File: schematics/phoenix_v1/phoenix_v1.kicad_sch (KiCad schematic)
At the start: 1 part, among them U1 ESP32-DevKitC

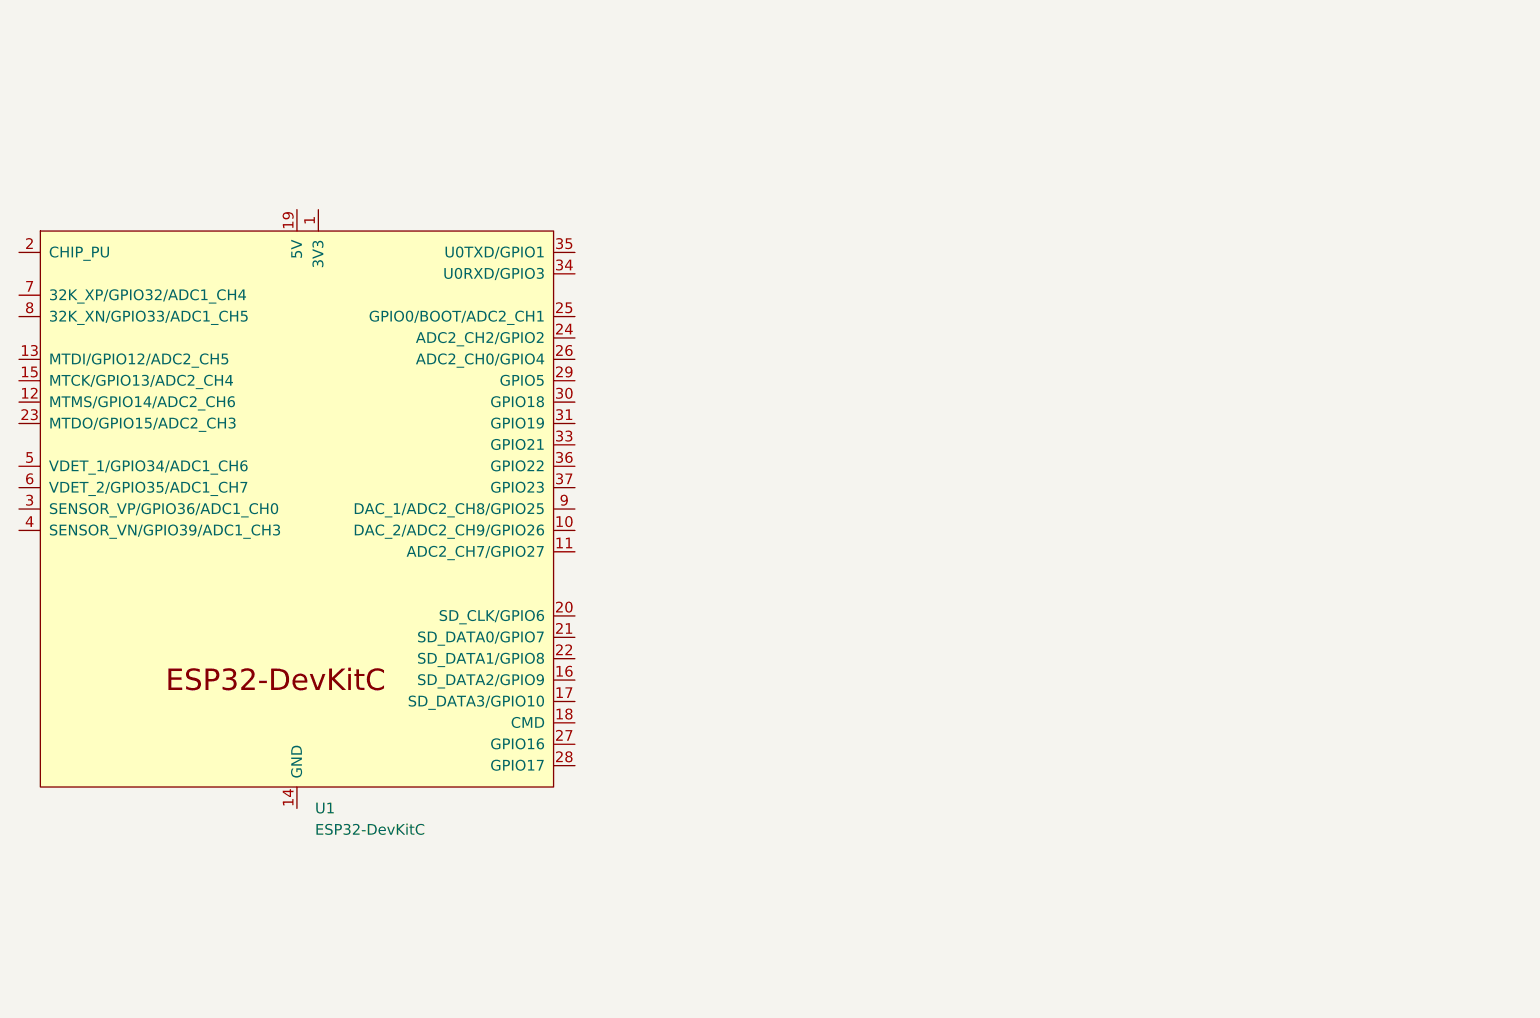
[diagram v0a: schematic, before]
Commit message: v1 schematic
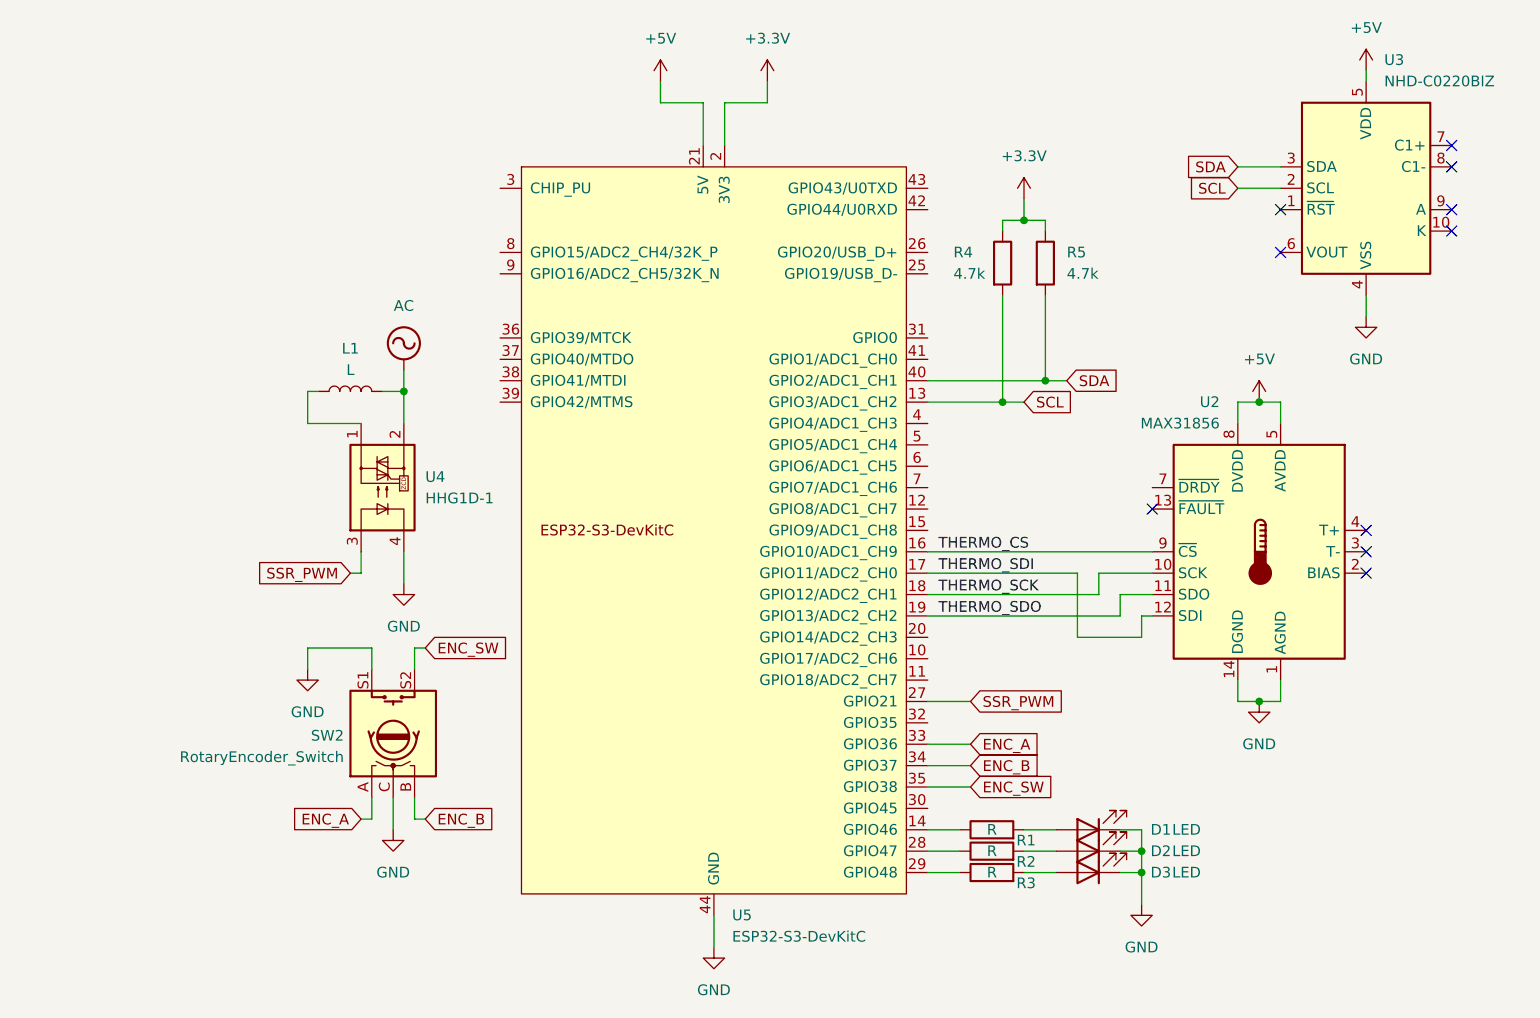
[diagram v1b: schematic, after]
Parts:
- removed U1: ESP32-DevKitC, PCM_Espressif:ESP32-DevKitC, symbol PCM_Espressif:ESP32-DevKitC
- added D1, D2, D3: LED, symbol Device:LED
- added L1: L, symbol Device:L
- added R1, R2, R3: R, symbol Device:R
- added R4, R5: 4.7k, symbol Device:R
- added SW2: RotaryEncoder_Switch, symbol Device:RotaryEncoder_Switch
- added U2: MAX31856, Package_SO:TSSOP-14_4.4x5mm_P0.65mm, symbol Sensor_Temperature:MAX31856
- added U3: NHD-C0220BIZ, Display:NHD-C0220BiZ, symbol Display_Character:NHD-C0220BIZ
- added U4: HHG1D-1, Relay_THT:Relay_NCR_HHG1D-1, symbol Relay_SolidState:HHG1D-1
- added U5: ESP32-S3-DevKitC, PCM_Espressif:ESP32-S3-DevKitC, symbol PCM_Espressif:ESP32-S3-DevKitC
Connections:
- new net: R1.1, U5.14 (GPIO46)
- new net: R2.1, U5.28 (GPIO47)
- new net: R3.1, U5.29 (GPIO48)
- new net: D3.2 (A), R3.2
- new net: D1.2 (A), R1.2
- new net: D2.2 (A), R2.2
- new net: L1.1, U4.1
- new net +3.3V: R4.1, R5.1, U5.1 (3V3), U5.2 (3V3)
- new net +5V: U2.5 (AVDD), U2.8 (DVDD), U3.5 (VDD), U5.21 (5V)
- new net AC: L1.2, U4.2
- new net ENC_A: SW2.A, U5.33 (GPIO36)
- new net ENC_B: SW2.B, U5.34 (GPIO37)
- new net ENC_SW: SW2.S2, U5.35 (GPIO38)
- new net GND: D1.1 (K), D2.1 (K), D3.1 (K), SW2.C, SW2.S1, U2.1 (AGND), U2.14 (DGND), U3.4 (VSS), U4.4, U5.22 (GND), U5.23 (GND), U5.24 (GND), U5.44 (GND)
- new net SCL: R4.2, U3.2 (SCL), U5.13 (GPIO3/ADC1_CH2)
- new net SDA: R5.2, U3.3 (SDA), U5.40 (GPIO2/ADC1_CH1)
- new net SSR_PWM: U4.3, U5.27 (GPIO21)
- new net THERMO_CS: U2.9 (~{CS}), U5.16 (GPIO10/ADC1_CH9)
- new net THERMO_SCK: U2.10 (SCK), U5.18 (GPIO12/ADC2_CH1)
- new net THERMO_SDI: U2.12 (SDI), U5.17 (GPIO11/ADC2_CH0)
- new net THERMO_SDO: U2.11 (SDO), U5.19 (GPIO13/ADC2_CH2)
- no-connect marks 0 -> 10
